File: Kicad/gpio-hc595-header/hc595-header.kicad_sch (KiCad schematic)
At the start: 7 parts, among them K1 GPIO IN, K2 GPIO OUT, K3 DATA OUTPUT, U1 74HC595-SOIC-16, U2 3M-SJ5376

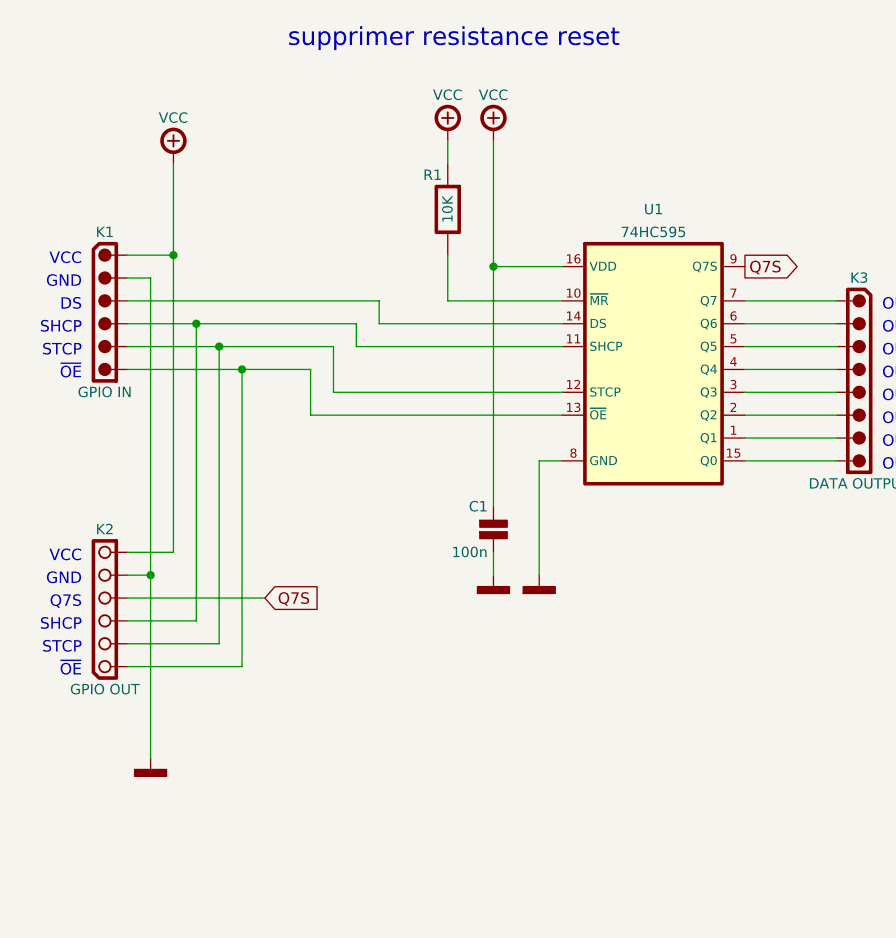
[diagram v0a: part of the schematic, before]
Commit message: Update
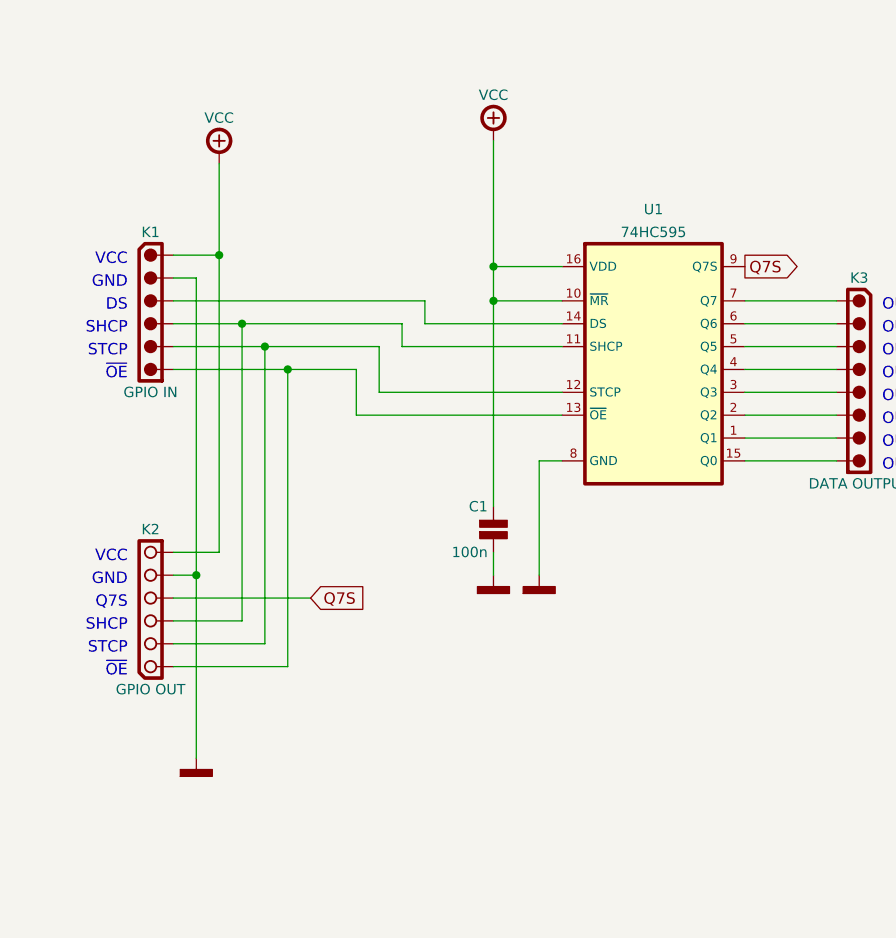
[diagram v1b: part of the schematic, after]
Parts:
- removed R1: 10K, tronixio:RESISTOR-1206, symbol tronixio:R-1210
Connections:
- net VCC: now also U1.10 (~{MR})
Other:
- note removed: "supprimer resistance reset"
- moved on the sheet: K1, K2
